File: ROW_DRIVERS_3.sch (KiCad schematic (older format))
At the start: 36 parts, among them Q132 DMG6602, Q133 DMG6602, Q134 SSM3K35AMFV, Q135 SSM3K35AMFV, Q136 SSM3K35AMFV, Q137 SSM3K35AMFV, Q138 DMG6602, Q139 DMG6602, Q140 SSM3K35AMFV, Q141 SSM3K35AMFV, Q142 SSM3K35AMFV, Q143 SSM3K35AMFV

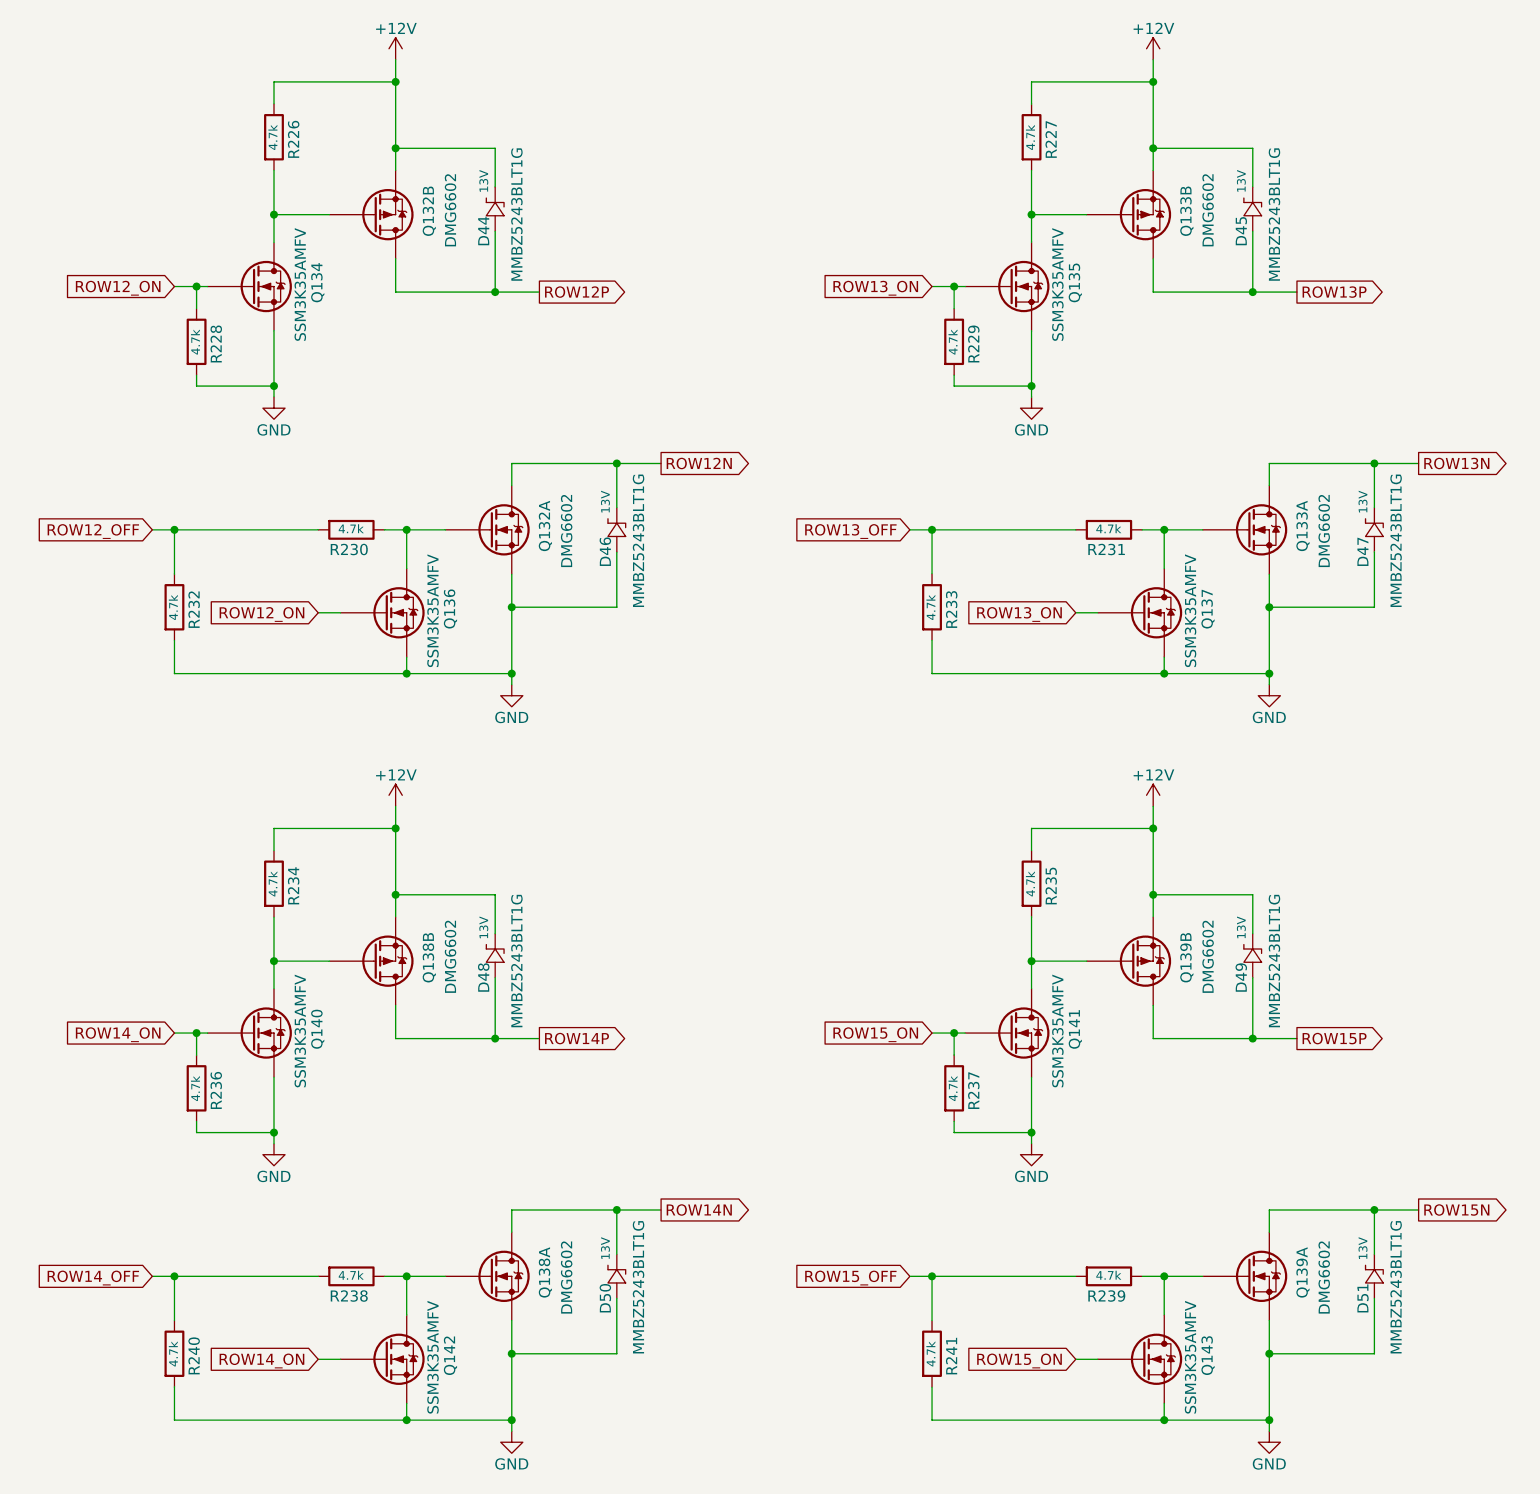
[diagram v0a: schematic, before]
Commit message: automated commit
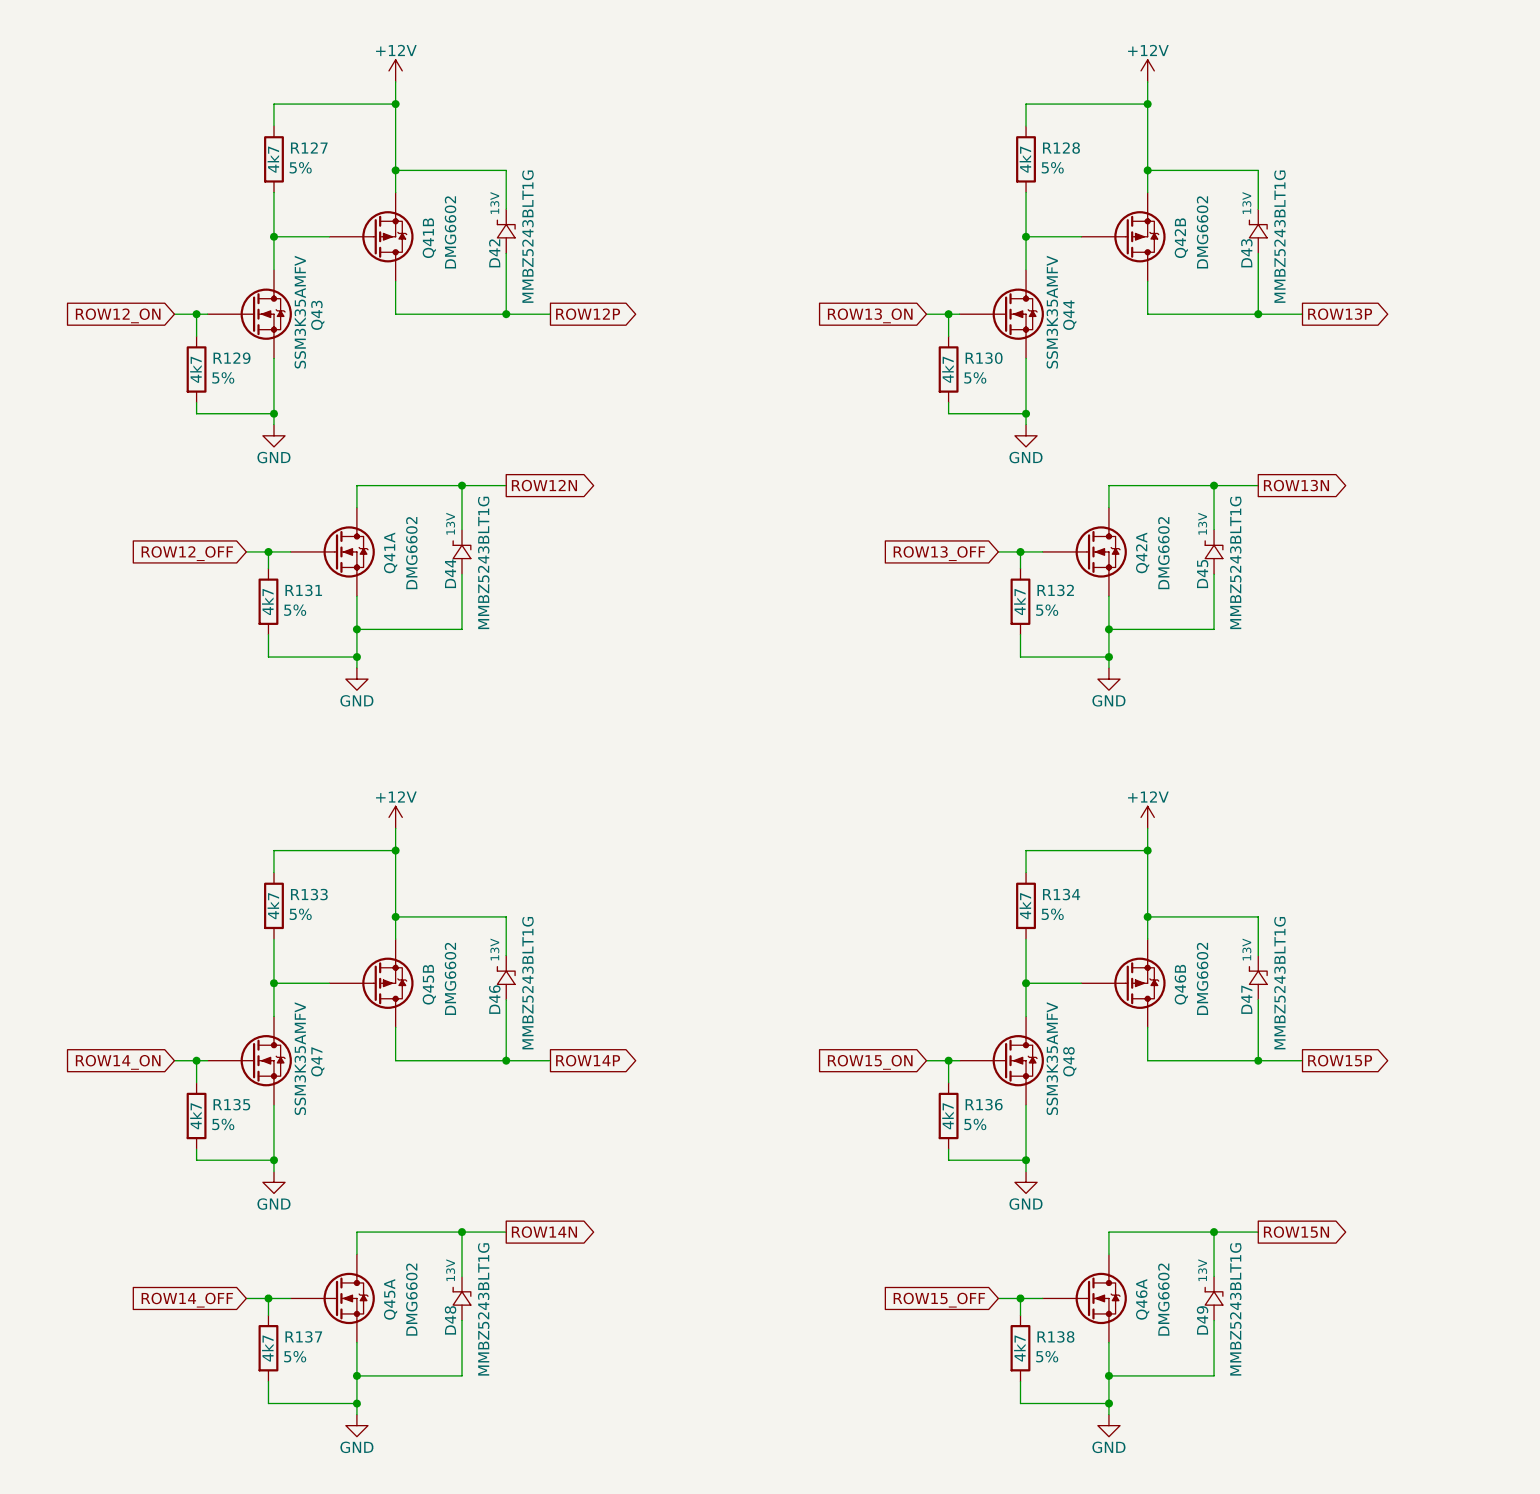
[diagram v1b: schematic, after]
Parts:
- removed D50, D51: MMBZ5243BLT1G, symbol custom:MMBZ5243BLT1G
- removed Q132, Q133, Q138, Q139: DMG6602, Package_TO_SOT_SMD:TSOT-23-6, symbol custom:DMG6602
- removed Q134, Q135, Q136, Q137, Q140, Q141, Q142, Q143: SSM3K35AMFV, symbol custom:SSM3K35AMFV
- removed R226, R227, R228, R229, R230, R231, R232, R233, R234, R235, R236, R237, R238, R239, R240, R241: CRG0603F4K7, Resistor_SMD:R_0603_1608Metric, symbol custom:CRG0603F4K7
- added D42, D43: MMBZ5243BLT1G, symbol custom:MMBZ5243BLT1G
- added Q41, Q42, Q45, Q46: DMG6602, Package_TO_SOT_SMD:TSOT-23-6, symbol custom:DMG6602
- added Q43, Q44, Q47, Q48: SSM3K35AMFV, symbol custom:SSM3K35AMFV
- added R127, R128, R129, R130, R131, R132, R133, R134, R135, R136, R137, R138: CRG0603F4K7, Resistor_SMD:R_0603_1608Metric, symbol custom:CRG0603F4K7
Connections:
- net +12V: now also D46.1 (K), D47.1 (K), D42.1 (K), D43.1 (K), Q41.2 (S), Q42.2 (S), Q45.2 (S), Q46.2 (S), R127.1, R128.1, R133.1, R134.1; no longer D44.1 (K), D45.1 (K), D48.1 (K), D49.1 (K)
- net GND: now also D44.2 (A), D45.2 (A), D48.2 (A), D49.2 (A), Q41.5 (S), Q42.5 (S), Q43.2 (S), Q44.2 (S), Q45.5 (S), Q46.5 (S), Q47.2 (S), Q48.2 (S), R129.2, R130.2, R131.2, R132.2, R135.2, R136.2, R137.2, R138.2; no longer D46.2 (A), D47.2 (A)
- net ROW12N: now also D44.1 (K), Q41.6 (D); no longer D46.1 (K)
- net ROW12P: now also D42.2 (A), Q41.4 (D); no longer D44.2 (A)
- net ROW12_OFF: now also Q41.1 (G), R131.1
- net ROW12_ON: now also Q43.1 (G), R129.1
- net ROW13N: now also D45.1 (K), Q42.6 (D); no longer D47.1 (K)
- net ROW13P: now also D43.2 (A), Q42.4 (D); no longer D45.2 (A)
- net ROW13_OFF: now also Q42.1 (G), R132.1
- net ROW13_ON: now also Q44.1 (G), R130.1
- net ROW14N: now also D48.1 (K), Q45.6 (D)
- net ROW14P: now also D46.2 (A), Q45.4 (D); no longer D48.2 (A)
- net ROW14_OFF: now also Q45.1 (G), R137.1
- net ROW14_ON: now also Q47.1 (G), R135.1
- net ROW15N: now also D49.1 (K), Q46.6 (D)
- net ROW15P: now also D47.2 (A), Q46.4 (D); no longer D49.2 (A)
- net ROW15_OFF: now also Q46.1 (G), R138.1
- net ROW15_ON: now also Q48.1 (G), R136.1
- new net: Q42.3 (G), Q44.3 (D), R128.2
- new net: Q46.3 (G), Q48.3 (D), R134.2
- new net: Q45.3 (G), Q47.3 (D), R133.2
- new net: Q41.3 (G), Q43.3 (D), R127.2
